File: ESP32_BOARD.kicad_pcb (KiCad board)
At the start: 4 copper layers, 36 x 63 mm, 70 parts, among them IC1 AP2112K-3.3, IC2 MPQ4420HGJ-Z, IC3 W25Q128JVSIQ, IC4 ESP32-S3R8, IC5 AW9364DNR, Q1 40MHz, SW1 TS-1010B-B-A, SW2 PTS810SJK250SMTRLFS, SW3 PTS810SJK250SMTRLFS

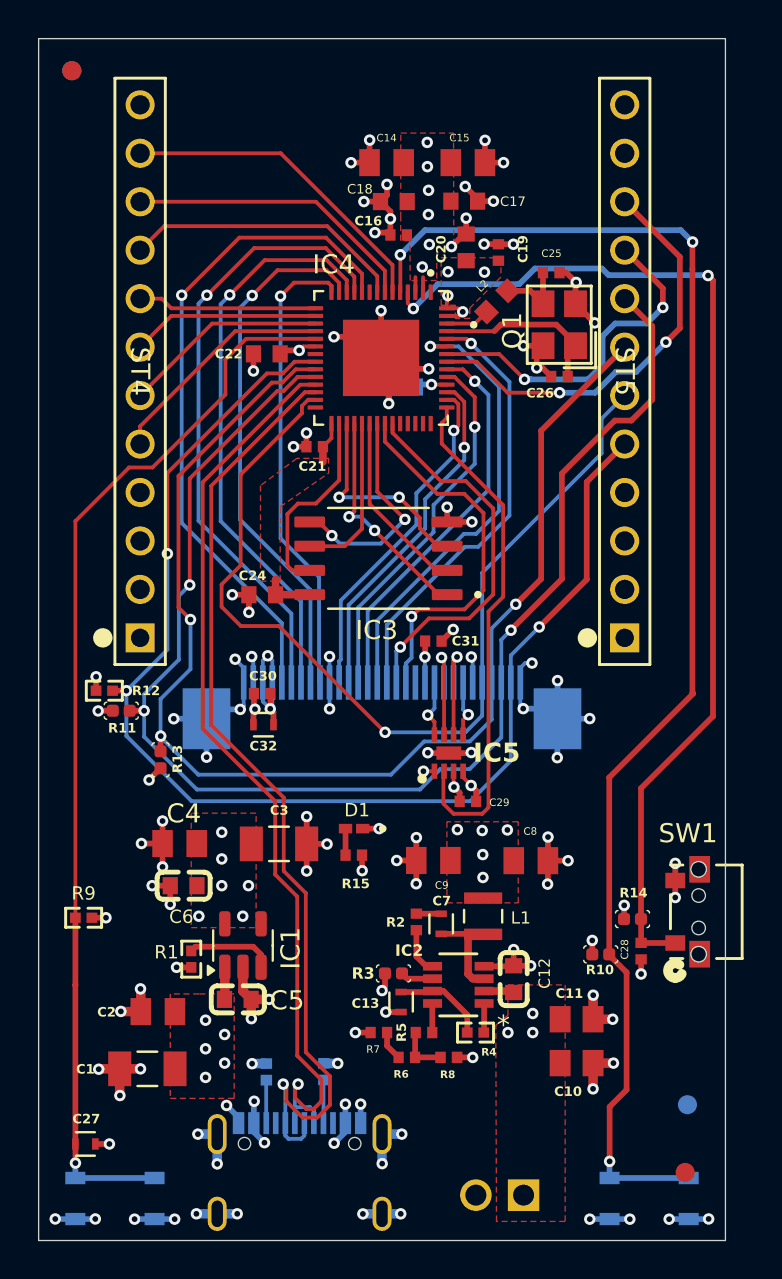
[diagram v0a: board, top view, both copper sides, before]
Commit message: Layout ready for export
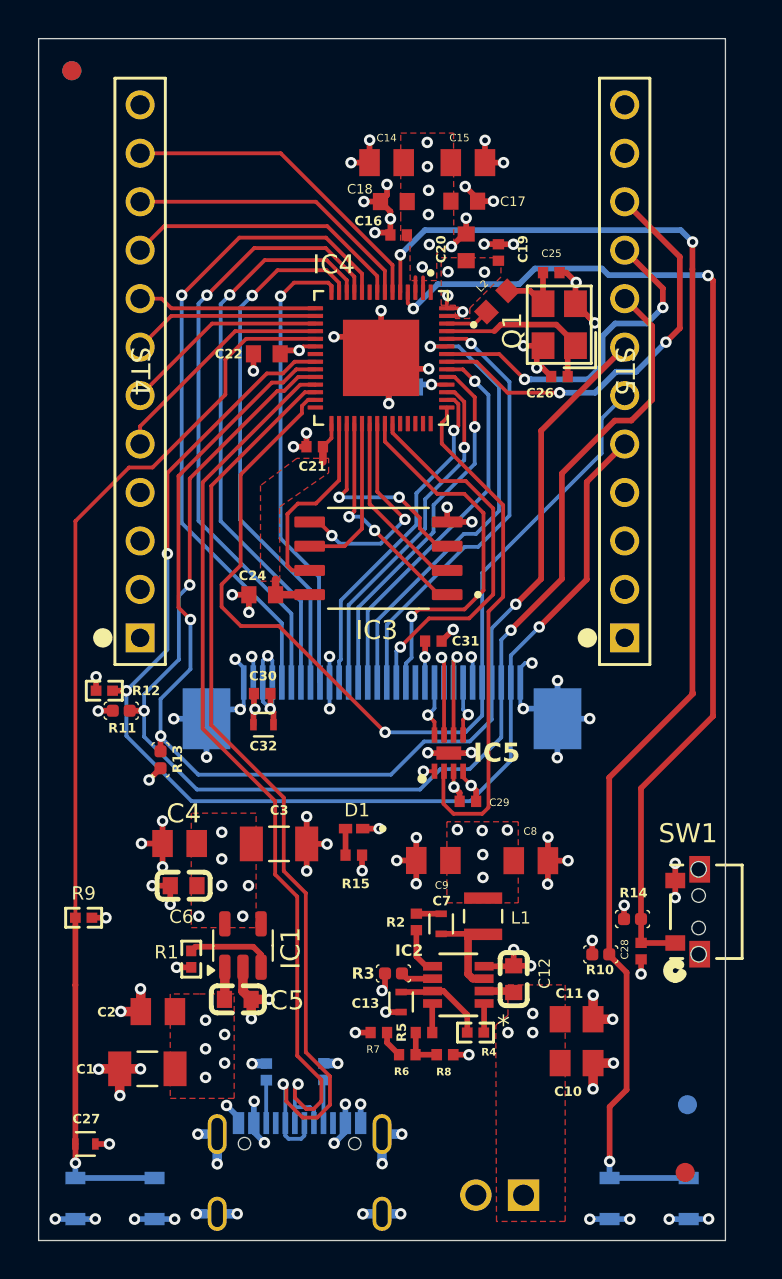
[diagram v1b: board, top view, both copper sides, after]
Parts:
- moved R8 0.24 mm to (98.7, 144.5)
- moved R6 0.14 mm to (96.7, 144.5)
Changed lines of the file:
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@@
 	(footprint "RC0402FR-0733KL:RESC1005X40N"
 		(layer "F.Cu")
-		(at 96.7 144.6 180)
+		(at 96.725 144.46 180)
 		(property "Reference" "R6"
 			(at 0.3 -0.88 0)
@@
 	(footprint "0402WGF1302TCE:RESC1005X40N"
 		(layer "F.Cu")
-		(at 98.9 144.6)
+		(at 98.7 144.46)
 		(property "Reference" "R8"
 			(at -0.06 0.9 0)
@@
 	)
 	(segment
-		(start 97.132 144.6)
-		(end 97.132 143.336)
+		(start 97.157 144.46)
+		(end 98.265 144.46)
 		(width 0.3)
 		(layer "F.Cu")
@@
 	)
 	(segment
-		(start 97.132 144.6)
-		(end 98.465 144.6)
+		(start 97.168 143.3)
+		(end 97.168 144.449)
 		(width 0.3)
 		(layer "F.Cu")
@@
 	)
 	(segment
-		(start 97.132 143.336)
-		(end 97.168 143.3)
+		(start 97.168 144.449)
+		(end 97.157 144.46)
 		(width 0.3)
 		(layer "F.Cu")
@@
 	)
 	(segment
-		(start 96.268 144.6)
-		(end 95.664 143.996)
+		(start 95.664 143.831)
+		(end 96.293 144.46)
 		(width 0.3)
 		(layer "F.Cu")
@@
 	)
 	(segment
-		(start 95.664 143.996)
-		(end 95.664 143.3)
+		(start 95.664 143.3)
+		(end 95.664 143.831)
 		(width 0.3)
 		(layer "F.Cu")
@@
 	)
 	(segment
-		(start 100.151429 144.6)
-		(end 100.154827 144.603398)
+		(start 99.951429 144.46)
+		(end 99.954827 144.463398)
 		(width 0.3)
 		(layer "F.Cu")
@@
 	)
 	(segment
-		(start 99.335 144.6)
-		(end 100.151429 144.6)
+		(start 99.135 144.46)
+		(end 99.951429 144.46)
 		(width 0.3)
 		(layer "F.Cu")
@@
 	)
 	(via
-		(at 100.154827 144.603398)
+		(at 99.954827 144.463398)
 		(size 0.6)
 		(drill 0.3)
@@
 	)
 	(segment
-		(start 89.92 109.66)
-		(end 85.32 114.26)
-		(width 0.2)
-		(layer "F.Cu")
-		(net 27)
-	)
-	(segment
-		(start 90.975 108.935)
-		(end 90.25 109.66)
+		(start 90.28 109.66)
+		(end 89.92 109.66)
 		(width 0.2)
 		(layer "F.Cu")
@@
 	)
 	(segment
+		(start 91.905 108.935)
+		(end 91.005 108.935)
+		(width 0.2)
+		(layer "F.Cu")
+		(net 27)
+	)
+	(segment
+		(start 91.005 108.935)
+		(end 90.28 109.66)
+		(width 0.2)
+		(layer "F.Cu")
+		(net 27)
+	)
+	(segment
 		(start 109.56 110.13)
 		(end 109.56 106.2701)
@@
 	)
 	(segment
-		(start 85.32 114.26)
-		(end 85.32 119.84)
+		(start 89.92 109.66)
+		(end 85.32 114.26)
 		(width 0.2)
 		(layer "F.Cu")
@@
 	)
 	(segment
-		(start 91.905 108.935)
-		(end 90.975 108.935)
-		(width 0.2)
+		(start 102.16 122.19)
+		(end 104.83 119.52)
+		(width 0.3)
 		(layer "F.Cu")
 		(net 27)
 	)
 	(segment
-		(start 90.25 109.66)
-		(end 89.92 109.66)
+		(start 85.32 114.26)
+		(end 85.32 119.84)
 		(width 0.2)
 		(layer "F.Cu")
@@
 	)
 	(segment
-		(start 102.16 122.19)
-		(end 104.83 119.52)
-		(width 0.3)
-		(layer "F.Cu")
-		(net 27)
-	)
-	(segment
 		(start 102.16 122.21)
 		(end 102.16 122.19)
@@
 	)
 	(segment
-		(start 84.73 121.02)
-		(end 85.36 121.65)
-		(width 0.2)
-		(layer "F.Cu")
-		(net 37)
-	)
-	(segment
 		(start 103.74 111.7499)
 		(end 103.74 119.52)
@@
 	)
 	(segment
-		(start 90.18 109.23)
-		(end 89.625678 109.23)
+		(start 84.73 114.125678)
+		(end 84.73 121.02)
 		(width 0.2)
 		(layer "F.Cu")
@@
 	)
 	(segment
-		(start 91.905 108.535)
-		(end 90.875 108.535)
-		(width 0.2)
+		(start 103.74 119.52)
+		(end 102.41 120.85)
+		(width 0.3)
 		(layer "F.Cu")
 		(net 37)
 	)
 	(segment
-		(start 84.73 114.125678)
-		(end 84.73 121.02)
-		(width 0.2)
+		(start 108.1199 107.37)
+		(end 103.74 111.7499)
+		(width 0.3)
 		(layer "F.Cu")
 		(net 37)
 	)
 	(segment
-		(start 103.74 119.52)
-		(end 102.41 120.85)
-		(width 0.3)
+		(start 89.625678 109.23)
+		(end 84.73 114.125678)
+		(width 0.2)
 		(layer "F.Cu")
 		(net 37)
 	)
 	(segment
-		(start 90.875 108.535)
-		(end 90.18 109.23)
+		(start 90.21 109.23)
+		(end 89.625678 109.23)
 		(width 0.2)
 		(layer "F.Cu")
@@
 	)
 	(segment
-		(start 108.1199 107.37)
-		(end 103.74 111.7499)
-		(width 0.3)
+		(start 91.905 108.535)
+		(end 90.905 108.535)
+		(width 0.2)
 		(layer "F.Cu")
 		(net 37)
@@
 	)
 	(segment
-		(start 89.625678 109.23)
-		(end 84.73 114.125678)
+		(start 84.73 121.02)
+		(end 85.36 121.65)
+		(width 0.2)
+		(layer "F.Cu")
+		(net 37)
+	)
+	(segment
+		(start 90.905 108.535)
+		(end 90.21 109.23)
 		(width 0.2)
 		(layer "F.Cu")
@@
 		(polygon
 			(pts
-				(xy 92.6 113.2) (xy 90.933334 113.2) (xy 89.03 114.6275) (xy 89.03 119.64) (xy 90.06 119.64) (xy 90.06 115.743024)
-				(xy 92.6 113.976067)
+				(xy 92.6 113.2) (xy 90.933334 113.2) (xy 89.03 114.6275) (xy 89.03 119.64) (xy 90.04 119.64) (xy 90.04 115.739979)
+				(xy 92.6 113.959109)
 			)
 		)
